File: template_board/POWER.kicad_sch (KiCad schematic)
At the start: 8 parts, among them U4 AZ1117-3.3

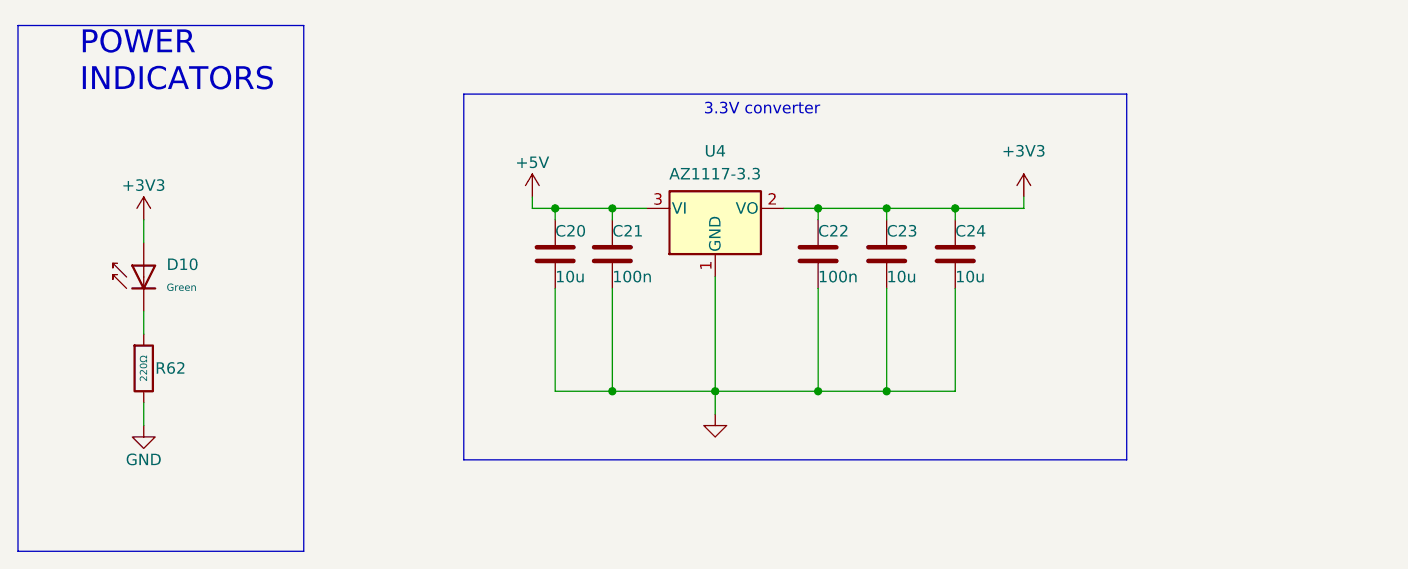
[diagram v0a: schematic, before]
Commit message: can transiver update
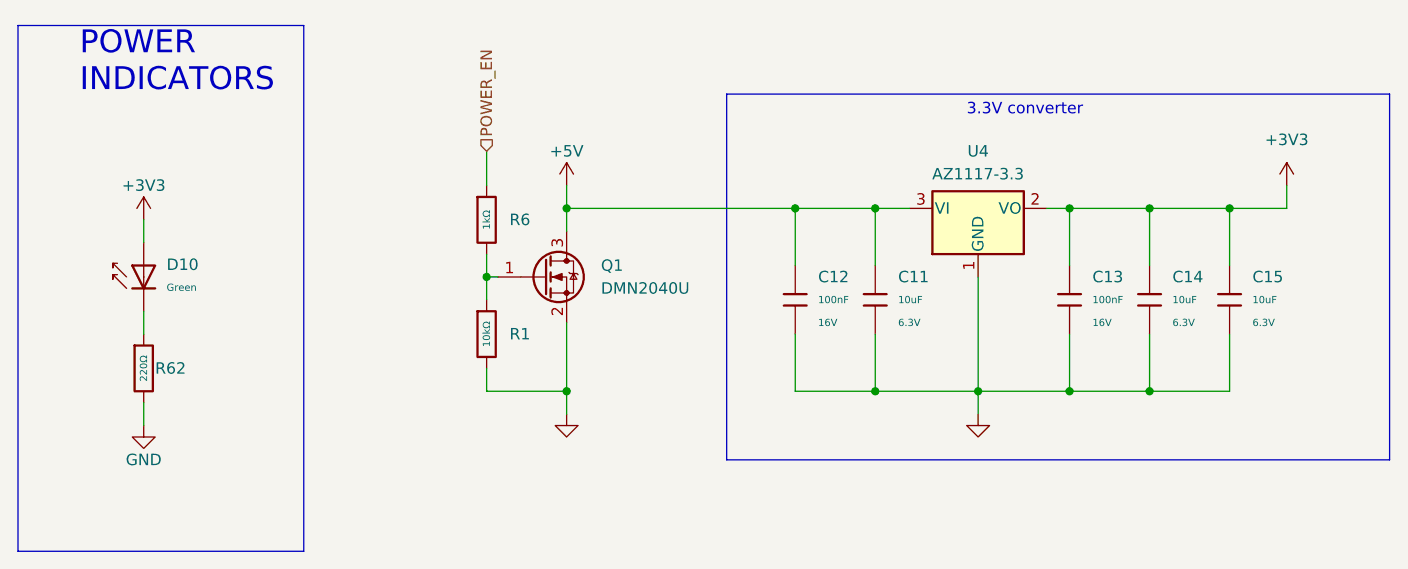
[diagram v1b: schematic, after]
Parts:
- removed C20, C23, C24: 10u, Capacitor_SMD:C_0805_2012Metric, symbol Device:C
- removed C21: 100n, Capacitor_SMD:C_0402_1005Metric, symbol Device:C
- removed C22: 100n, Capacitor_SMD:C_0603_1608Metric, symbol Device:C
- added C11, C14, C15: 10uF, PCM_JLCPCB:C_0402, symbol PCM_JLCPCB-Capacitors:0402,10uF
- added C12, C13: 100nF, PCM_JLCPCB:C_0402, symbol PCM_JLCPCB-Capacitors:0402,100nF
- added Q1: DMN2040U, Package_TO_SOT_SMD:SOT-23, symbol Transistor_FET:DMN2040U
- added R1: 10kΩ, PCM_JLCPCB:R_0402, symbol PCM_JLCPCB-Resistors:0402,10kΩ
- added R6: 1kΩ, PCM_JLCPCB:R_0402, symbol PCM_JLCPCB-Resistors:0402,1kΩ
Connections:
- net +3V3: now also C13.1, C14.1, C15.1
- net +5V: now also C11.1, C12.1, Q1.3 (D)
- net GND: now also C11.2, C12.2, C13.2, C14.2, C15.2, Q1.2 (S), R1.2
- new net: Q1.1 (G), R1.1, R6.2
- new net POWER_EN: R6.1
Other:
- moved on the sheet: U4
